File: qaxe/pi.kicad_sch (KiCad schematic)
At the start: 45 parts, among them J4 Conn_01x02, J5 Conn_01x02, J5 SWD, J6 USB_C_Receptacle_USB2.0, M2 Fan_4pin, SW1 boot, U13 TMP1075, U35 STM32L151CCT6, U37 TXU0101, U39 TXU0101, X1 8MHz

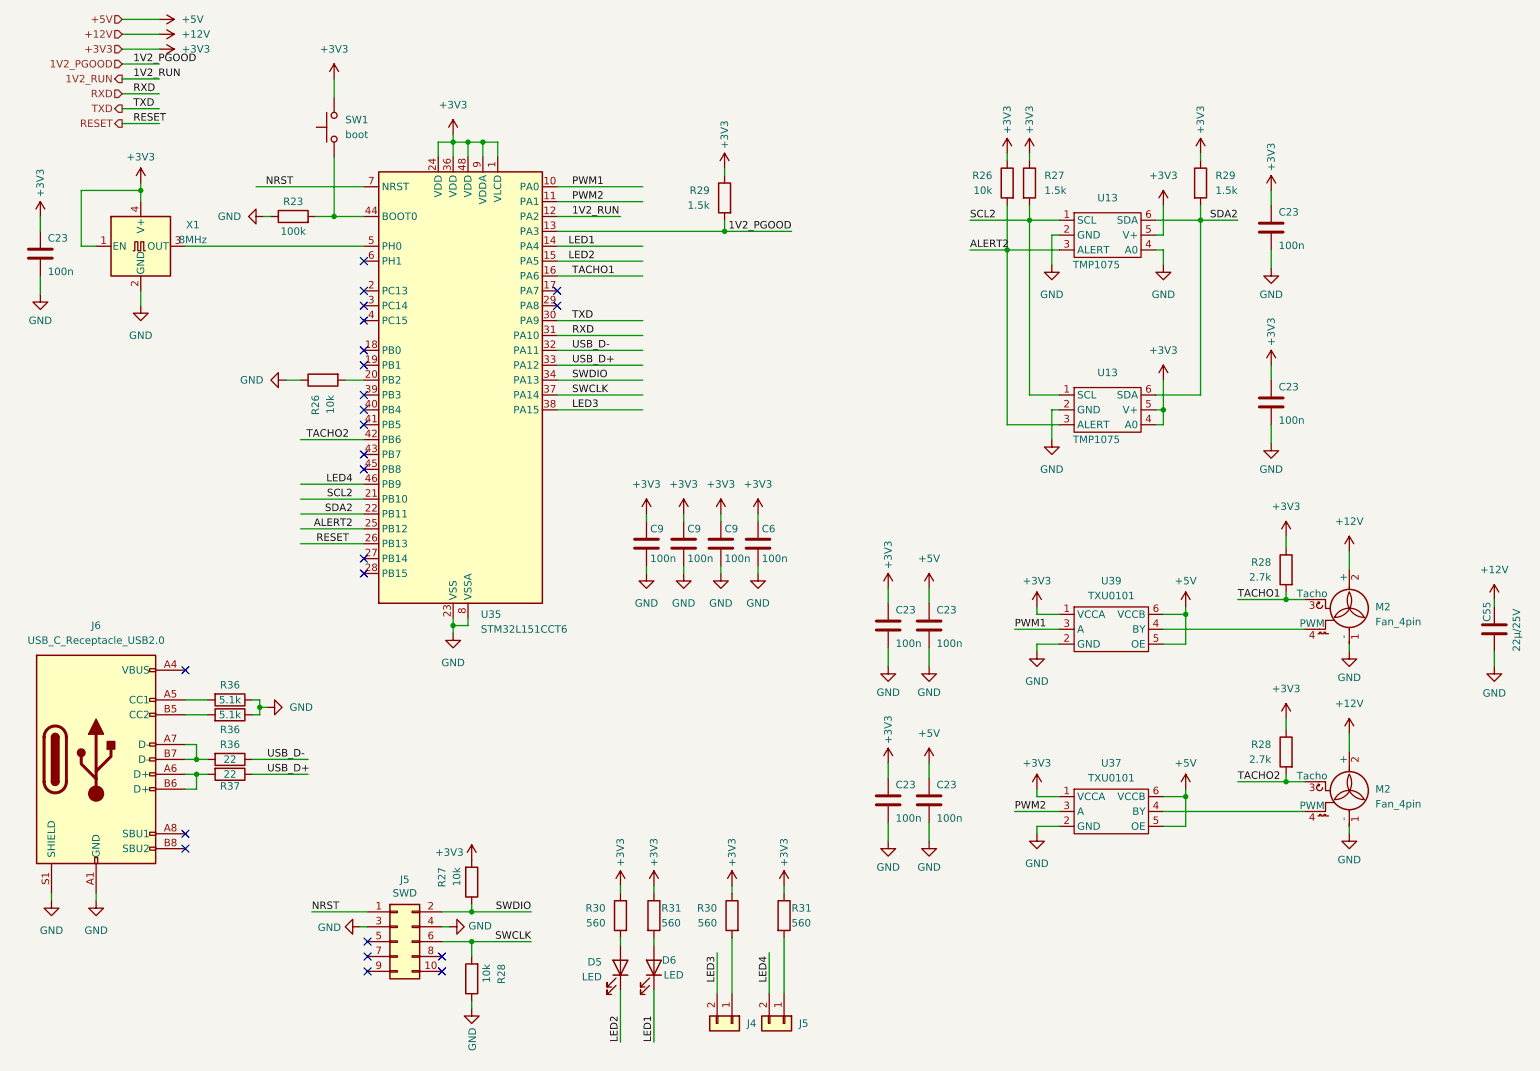
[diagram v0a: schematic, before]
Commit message: 1368 support
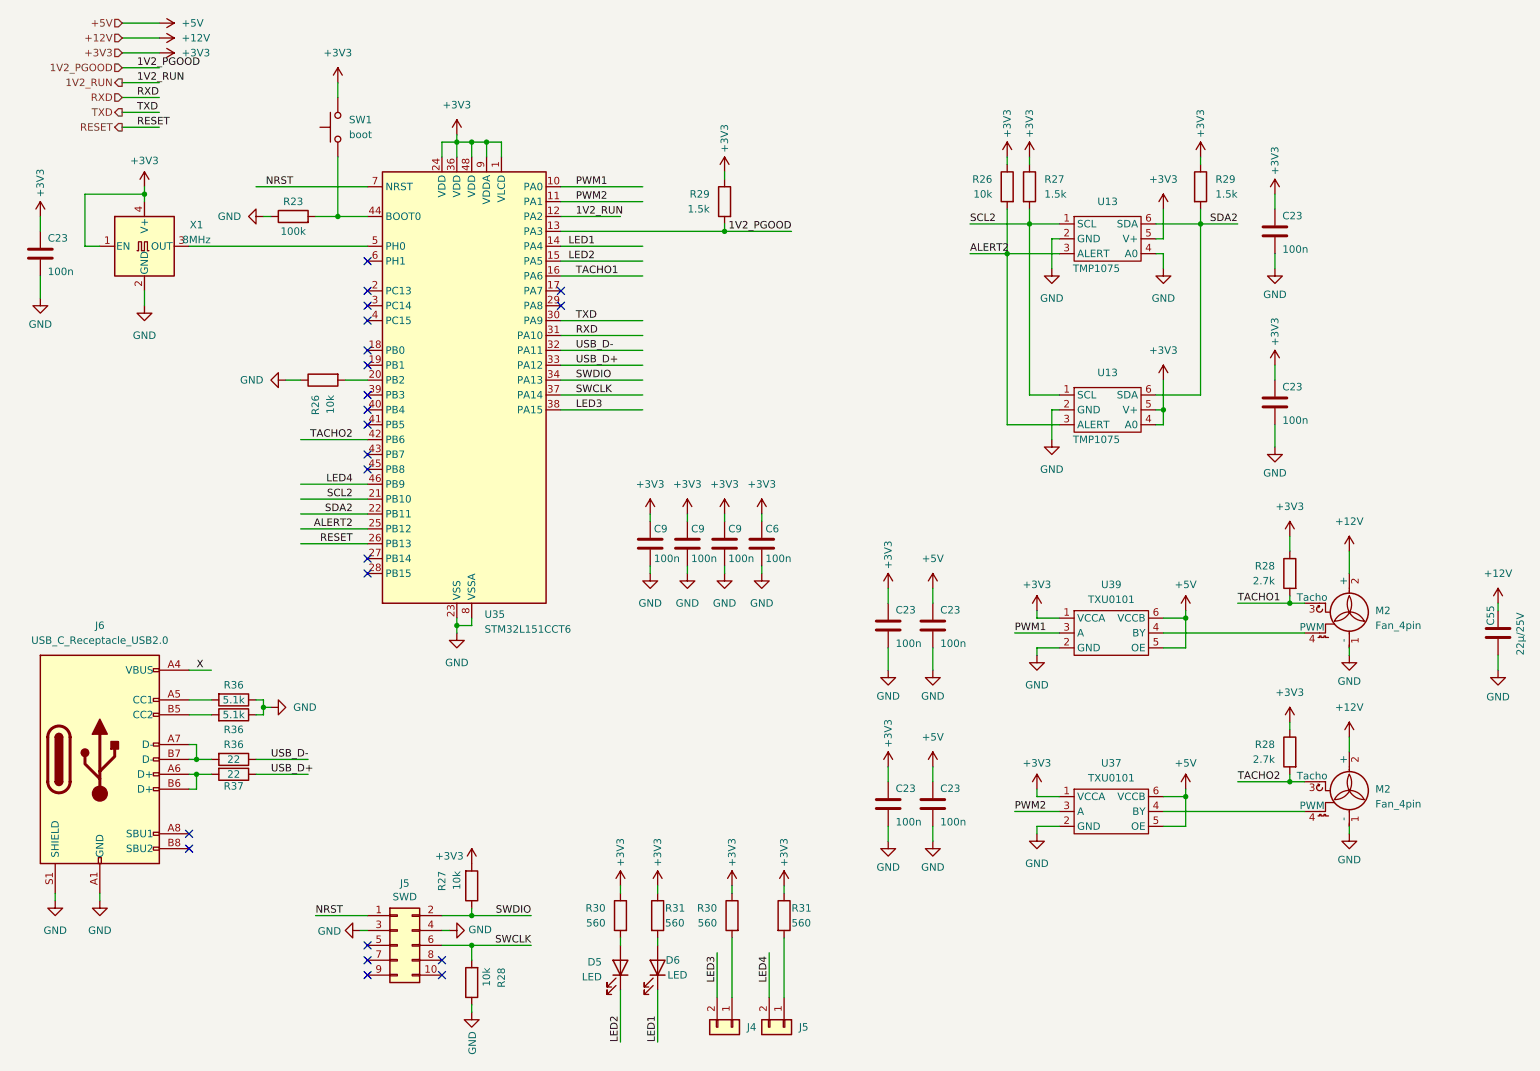
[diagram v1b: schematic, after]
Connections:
- net X: now reaches J6.A4 (VBUS), J6.A9 (VBUS), J6.B4 (VBUS), J6.B9 (VBUS)
- no-connect marks 23 -> 22
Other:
- moved on the sheet: C23, C55, C6, C9, D6, J4, J5, J6, M2, R26, R27, R28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
